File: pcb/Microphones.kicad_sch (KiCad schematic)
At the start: 40 parts, among them J16 Conn_02x01, U1 AD8426ACPZ-R7, U2 AD8426ACPZ-R7, U3 LT1790ACS6-1.25

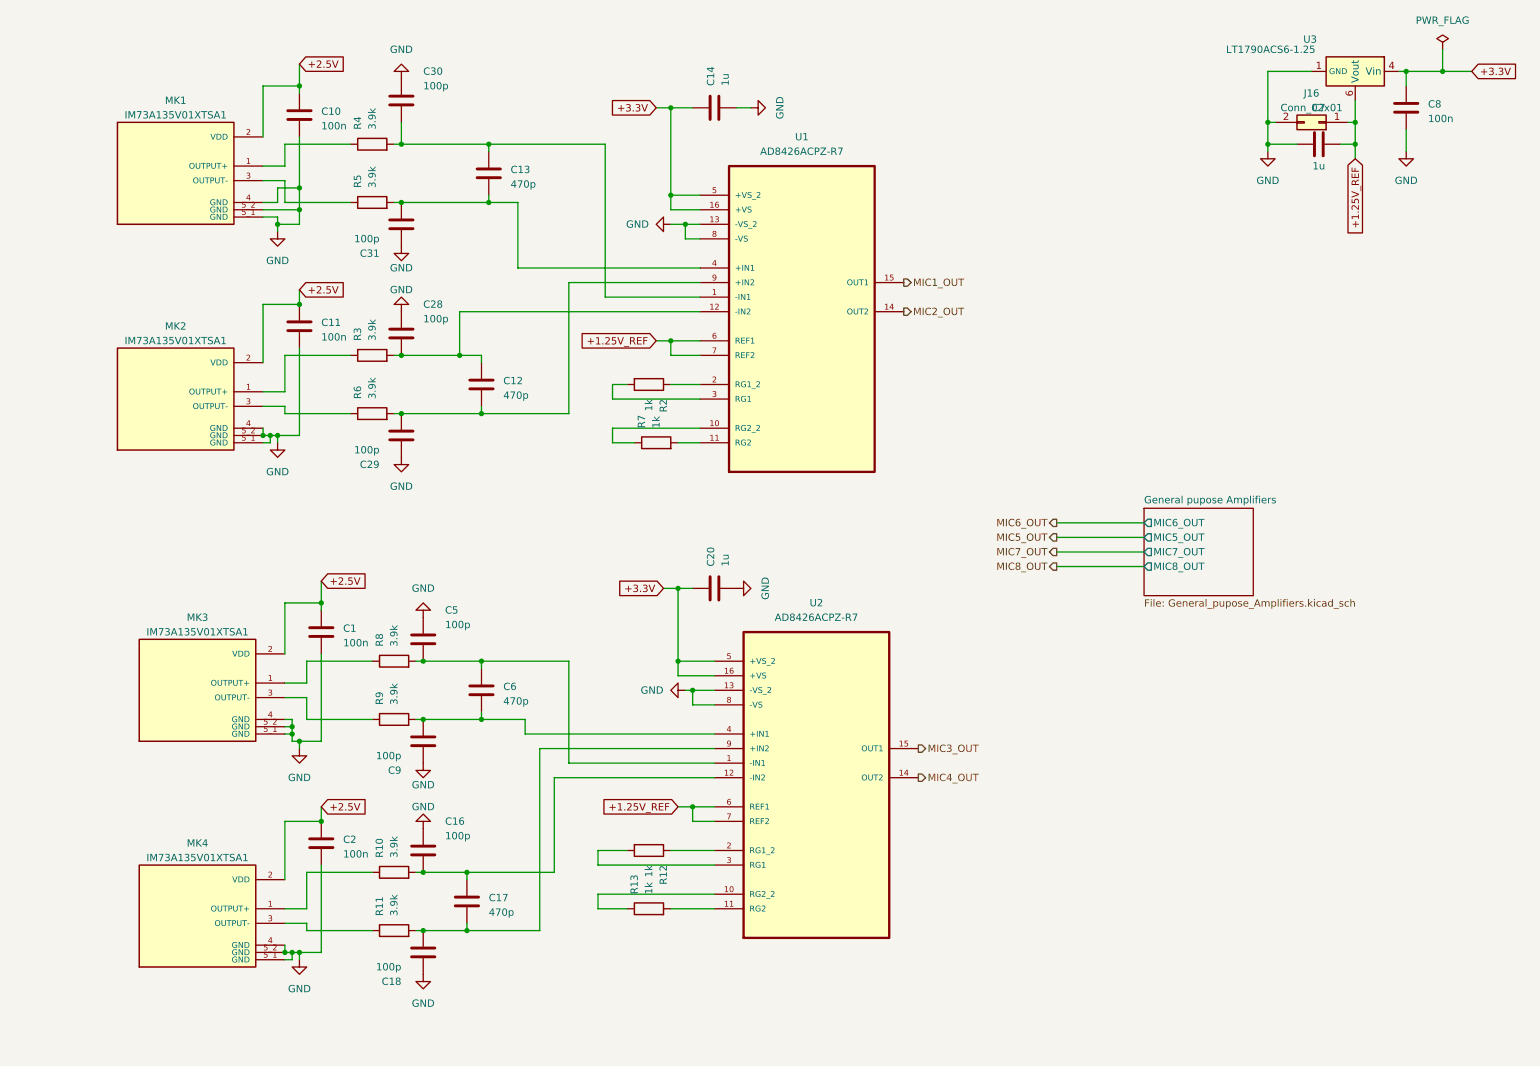
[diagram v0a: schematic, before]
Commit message: Polishin pt1
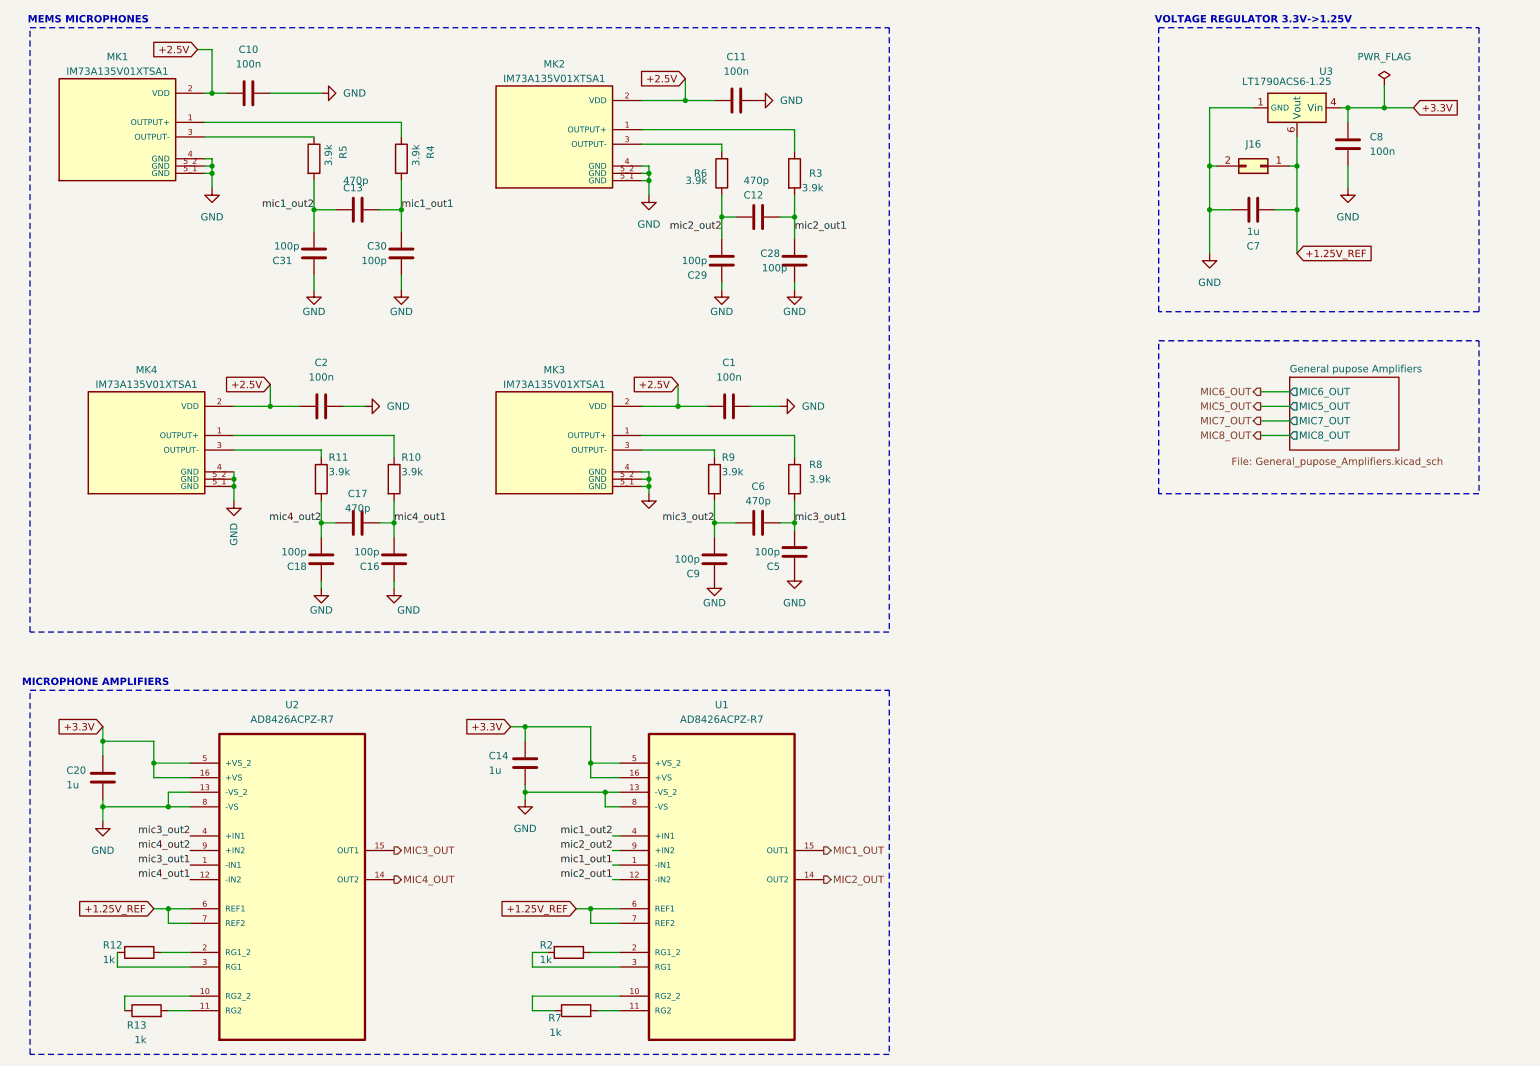
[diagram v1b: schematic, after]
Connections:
- net at MK2.3 (OUTPUT-): now also R6.2; no longer R6.1
- net mic2_out2: now reaches C12.2, C29.2, U1.9 (+IN2)
- net mic2_out2: now also R6.1; no longer R6.2
- net mic3_out1: now reaches C5.2, C6.1, R8.2, U2.1 (-IN1)
- net mic4_out1: now reaches C16.2, R10.2, U2.12 (-IN2)
- net mic4_out1: now also C17.2; no longer C17.1
- net mic3_out2: now reaches C6.2, C9.2, R9.2, U2.4 (+IN1)
- net mic4_out2: now reaches C18.2, R11.2, U2.9 (+IN2)
- net mic4_out2: now also C17.1; no longer C17.2
- net mic2_out1: now reaches C12.1, C28.2, R3.2, U1.12 (-IN2)
- net mic1_out2: now reaches C13.2, C31.2, R5.2, U1.4 (+IN1)
- net mic1_out1: now reaches C13.1, C30.2, R4.2, U1.1 (-IN1)
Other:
- note added: "MEMS MICROPHONES"
- note added: "MICROPHONE AMPLIFIERS"
- note added: "VOLTAGE REGULATOR 3.3V->1.25V"
- company: (none) -> Infineon Technologies
- title: (none) -> SensEdu 0.7
- moved on the sheet: C1, C10, C11, C12, C13, C14, C16, C17, C18, C2, C20, C28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
